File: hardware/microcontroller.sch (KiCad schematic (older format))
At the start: 8 parts, among them J1 Conn_02x05_Odd_Even, U1 ESP-WROOM-32

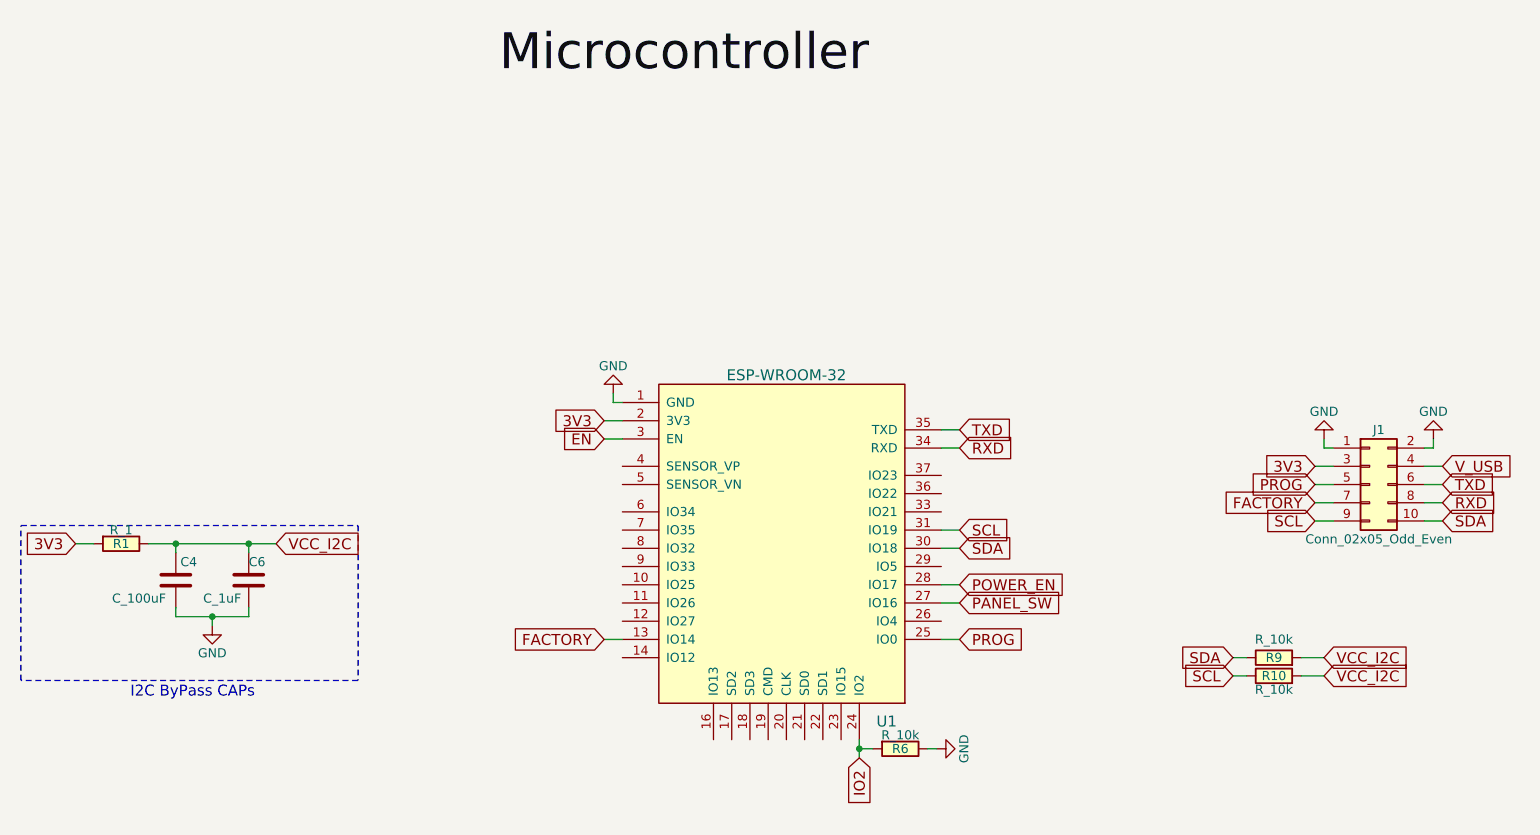
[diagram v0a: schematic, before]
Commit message: update
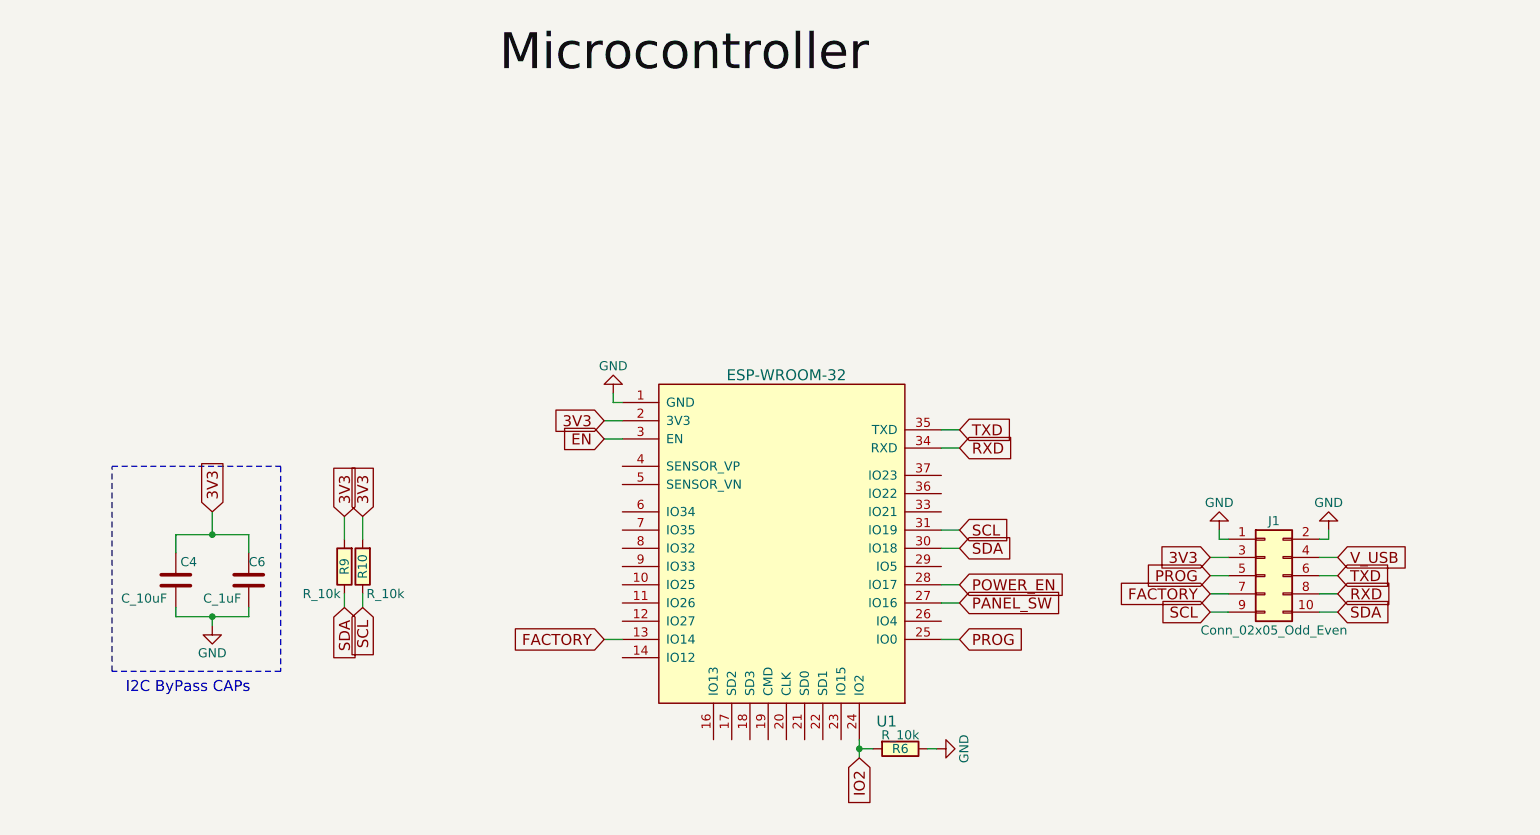
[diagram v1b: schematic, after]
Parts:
- removed C4: C_100uF, Capacitors_SMD:C_1206_HandSoldering, symbol C_100uF
- removed R1: R_1, Resistors_SMD:R_0603_HandSoldering, symbol R_1
- added C4: C_10uF, Capacitors_SMD:C_0603_HandSoldering, symbol C_10uF
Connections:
- net VCC_I2C is gone; now on net 3V3: C6.1, R10.2, R9.2
- net 3V3: now also C4.1
- net GND: now also C4.2
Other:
- moved on the sheet: J1, R10, R9
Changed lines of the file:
@@
 L GND #PWR02
 U 1 1 590979B0
-P 8725 3000
-F 0 "#PWR02" H 8725 2750 50  0001 C CNN
-F 1 "GND" H 8725 2850 50  0000 C CNN
-F 2 "" H 8725 3000 50  0000 C CNN
-F 3 "" H 8725 3000 50  0000 C CNN
-	1    8725 3000
-	-1   0    0    1
-$EndComp
-Text GLabel 8675 3150 0    60   Input ~ 0
-3V3
-Text GLabel 9375 3350 2    60   Input ~ 0
+P 8150 3500
+F 0 "#PWR02" H 8150 3250 50  0001 C CNN
+F 1 "GND" H 8150 3350 50  0000 C CNN
+F 2 "" H 8150 3500 50  0000 C CNN
+F 3 "" H 8150 3500 50  0000 C CNN
+	1    8150 3500
+	-1   0    0    1
+$EndComp
+Text GLabel 8100 3650 0    60   Input ~ 0
+3V3
+Text GLabel 8800 3850 2    60   Input ~ 0
 RXD
-Text GLabel 9375 3250 2    60   Input ~ 0
+Text GLabel 8800 3750 2    60   Input ~ 0
 TXD
-Text GLabel 9375 3150 2    60   Input ~ 0
+Text GLabel 8800 3650 2    60   Input ~ 0
 V_USB
 $Comp
 L GND #PWR03
 U 1 1 590979B2
-P 9325 3000
-F 0 "#PWR03" H 9325 2750 50  0001 C CNN
-F 1 "GND" H 9325 2850 50  0000 C CNN
-F 2 "" H 9325 3000 50  0000 C CNN
-F 3 "" H 9325 3000 50  0000 C CNN
-	1    9325 3000
-	-1   0    0    1
-$EndComp
-Wire Wire Line
-	9325 3050 9325 3000
-Wire Wire Line
-	9275 3050 9325 3050
-Wire Wire Line
-	8725 3050 8775 3050
-Wire Wire Line
-	8725 3000 8725 3050
-Wire Wire Line
-	9275 3150 9375 3150
-Wire Wire Line
-	9375 3350 9275 3350
-Wire Wire Line
-	9275 3250 9375 3250
-Wire Wire Line
-	8675 3150 8775 3150
+P 8750 3500
+F 0 "#PWR03" H 8750 3250 50  0001 C CNN
+F 1 "GND" H 8750 3350 50  0000 C CNN
+F 2 "" H 8750 3500 50  0000 C CNN
+F 3 "" H 8750 3500 50  0000 C CNN
+	1    8750 3500
+	-1   0    0    1
+$EndComp
+Wire Wire Line
+	8750 3550 8750 3500
+Wire Wire Line
+	8700 3550 8750 3550
+Wire Wire Line
+	8150 3550 8200 3550
+Wire Wire Line
+	8150 3500 8150 3550
+Wire Wire Line
+	8700 3650 8800 3650
+Wire Wire Line
+	8800 3850 8700 3850
+Wire Wire Line
+	8700 3750 8800 3750
+Wire Wire Line
+	8100 3650 8200 3650
 Wire Wire Line
 	6625 3800 6725 3800
@@
 $EndComp
 $Comp
-L C_100uF C4
-U 1 1 59C55B04
-P 2425 3775
-F 0 "C4" H 2450 3875 50  0000 L CNN
-F 1 "C_100uF" H 2075 3675 50  0000 L CNN
-F 2 "Capacitors_SMD:C_1206_HandSoldering" H 2525 4075 50  0001 C CNN
-F 3 "https://www.digikey.com/product-detail/en/tdk-corporation/C3216X5R1A107M160AC/445-6007-1-ND/2444048" H 2425 3525 50  0001 C CNN
-F 4 "C3216X5R1A107M160AC" H 2550 3975 60  0001 C CNN "Part Number"
-	1    2425 3775
-	1    0    0    -1
-$EndComp
-$Comp
 L GND #PWR04
 U 1 1 59C55B05
@@
 	1    0    0    -1
 $EndComp
-Text GLabel 1875 3575 0    60   Input ~ 0
-3V3
-Text GLabel 2975 3575 2    60   Input ~ 0
-VCC_I2C
-Wire Wire Line
-	1875 3575 1975 3575
-Wire Wire Line
-	2275 3575 2975 3575
-Wire Wire Line
-	2425 3575 2425 3625
-Wire Wire Line
-	2825 3575 2825 3625
-Connection ~ 2425 3575
-Connection ~ 2825 3575
+Text GLabel 2625 3400 1    60   Input ~ 0
+3V3
 Wire Wire Line
 	2425 3925 2425 3975
@@
 	2625 4025 2625 3975
 Connection ~ 2625 3975
-Text Notes 2175 4425 0    60   ~ 0
+Text Notes 2150 4400 0    60   ~ 0
 I2C ByPass CAPs
-Wire Notes Line
-	3425 3475 3425 4325
-Wire Notes Line
-	3425 4325 1575 4325
-Wire Notes Line
-	1575 4325 1575 3475
-Wire Notes Line
-	1575 3475 3425 3475
-Text GLabel 8675 3250 0    60   Input ~ 0
+Text GLabel 8100 3750 0    60   Input ~ 0
 PROG
-Text GLabel 8675 3350 0    60   Input ~ 0
+Text GLabel 8100 3850 0    60   Input ~ 0
 FACTORY
 Wire Wire Line
-	8675 3350 8775 3350
-Wire Wire Line
-	8675 3250 8775 3250
+	8100 3850 8200 3850
+Wire Wire Line
+	8100 3750 8200 3750
 $Comp
 L R_10k R6
@@
 Text GLabel 4775 3000 0    60   Input ~ 0
 EN
-Text GLabel 8675 3450 0    60   Input ~ 0
+Text GLabel 8100 3950 0    60   Input ~ 0
 SCL
-Text GLabel 9375 3450 2    60   Input ~ 0
+Text GLabel 8800 3950 2    60   Input ~ 0
 SDA
 Wire Wire Line
-	8675 3450 8775 3450
-Wire Wire Line
-	9275 3450 9375 3450
+	8100 3950 8200 3950
+Wire Wire Line
+	8700 3950 8800 3950
 Text GLabel 6725 3900 2    60   Input ~ 0
 PANEL_SW
@@
 L Conn_02x05_Odd_Even J1
 U 1 1 59C6C1C0
-P 8975 3250
-F 0 "J1" H 9025 3550 50  0000 C CNN
-F 1 "Conn_02x05_Odd_Even" H 9025 2950 50  0000 C CNN
-F 2 "Pin_Headers:Pin_Header_Straight_2x05_Pitch2.54mm" H 8975 3250 50  0001 C CNN
-F 3 "" H 8975 3250 50  0001 C CNN
-	1    8975 3250
-	1    0    0    -1
-$EndComp
-Text GLabel 8225 4300 0    60   Input ~ 0
+P 8400 3750
+F 0 "J1" H 8450 4050 50  0000 C CNN
+F 1 "Conn_02x05_Odd_Even" H 8450 3450 50  0000 C CNN
+F 2 "Pin_Headers:Pin_Header_Straight_2x05_Pitch2.54mm" H 8400 3750 50  0001 C CNN
+F 3 "" H 8400 3750 50  0001 C CNN
+	1    8400 3750
+	1    0    0    -1
+$EndComp
+Text GLabel 3450 3925 3    60   Input ~ 0
 SCL
-Text GLabel 8225 4200 0    60   Input ~ 0
+Text GLabel 3350 3925 3    60   Input ~ 0
 SDA
 $Comp
 L R_10k R10
 U 1 1 59C83F25
-P 8450 4300
-F 0 "R10" V 8450 4300 50  0000 C CNN
-F 1 "R_10k" V 8375 4300 50  0000 C CNN
-F 2 "Resistors_SMD:R_0603_HandSoldering" V 8380 4300 50  0001 C CNN
-F 3 "https://www.digikey.com/product-detail/en/yageo/RC0603JR-0710KL/311-10KGRCT-ND/729647" V 8530 4300 50  0001 C CNN
-F 4 "RC0603JR-0710KL" V 8630 4400 60  0001 C CNN "Part Number"
-	1    8450 4300
-	0    -1   -1   0
+P 3450 3700
+F 0 "R10" V 3450 3700 50  0000 C CNN
+F 1 "R_10k" H 3325 3850 50  0000 C CNN
+F 2 "Resistors_SMD:R_0603_HandSoldering" V 3380 3700 50  0001 C CNN
+F 3 "https://www.digikey.com/product-detail/en/yageo/RC0603JR-0710KL/311-10KGRCT-ND/729647" V 3530 3700 50  0001 C CNN
+F 4 "RC0603JR-0710KL" V 3630 3800 60  0001 C CNN "Part Number"
+	1    3450 3700
+	-1   0    0    1
 $EndComp
 $Comp
 L R_10k R9
 U 1 1 59C83F7C
-P 8450 4200
-F 0 "R9" V 8450 4200 50  0000 C CNN
-F 1 "R_10k" V 8550 4200 50  0000 C CNN
-F 2 "Resistors_SMD:R_0603_HandSoldering" V 8380 4200 50  0001 C CNN
-F 3 "https://www.digikey.com/product-detail/en/yageo/RC0603JR-0710KL/311-10KGRCT-ND/729647" V 8530 4200 50  0001 C CNN
-F 4 "RC0603JR-0710KL" V 8630 4300 60  0001 C CNN "Part Number"
-	1    8450 4200
-	0    -1   -1   0
-$EndComp
-Wire Wire Line
-	8300 4300 8225 4300
-Wire Wire Line
-	8225 4200 8300 4200
-Wire Wire Line
-	8600 4200 8725 4200
-Wire Wire Line
-	8725 4300 8600 4300
-Text GLabel 8725 4200 2    60   Input ~ 0
-VCC_I2C
-Text GLabel 8725 4300 2    60   Input ~ 0
-VCC_I2C
-$Comp
-L R_1 R1
-U 1 1 59E3C91A
-P 2125 3575
-F 0 "R1" V 2125 3575 50  0000 C CNN
-F 1 "R_1" V 2050 3575 50  0000 C CNN
-F 2 "Resistors_SMD:R_0603_HandSoldering" V 2055 3575 50  0001 C CNN
-F 3 "https://www.digikey.com/product-detail/en/stackpole-electronics-inc/RNCP0603FTD1R00/RNCP0603FTD1R00CT-ND/2240411" V 2205 3575 50  0001 C CNN
-F 4 "RNCP0603FTD1R00" V 2305 3675 60  0001 C CNN "Part Number"
-	1    2125 3575
-	0    1    1    0
-$EndComp
+P 3350 3700
+F 0 "R9" V 3350 3700 50  0000 C CNN
+F 1 "R_10k" H 3475 3850 50  0000 C CNN
+F 2 "Resistors_SMD:R_0603_HandSoldering" V 3280 3700 50  0001 C CNN
+F 3 "https://www.digikey.com/product-detail/en/yageo/RC0603JR-0710KL/311-10KGRCT-ND/729647" V 3430 3700 50  0001 C CNN
+F 4 "RC0603JR-0710KL" V 3530 3800 60  0001 C CNN "Part Number"
+	1    3350 3700
+	-1   0    0    1
+$EndComp
+Wire Wire Line
+	3450 3850 3450 3925
+Wire Wire Line
+	3350 3925 3350 3850
+Wire Wire Line
+	3350 3550 3350 3425
+Wire Wire Line
+	3450 3425 3450 3550
+Text GLabel 3350 3425 1    60   Input ~ 0
+3V3
+Text GLabel 3450 3425 1    60   Input ~ 0
+3V3
+$Comp
+L C_10uF C4
+U 1 1 5A10664F
+P 2425 3775
+F 0 "C4" H 2450 3875 50  0000 L CNN
+F 1 "C_10uF" H 2125 3675 50  0000 L CNN
+F 2 "Capacitors_SMD:C_0603_HandSoldering" H 2525 4075 50  0001 C CNN
+F 3 "https://www.digikey.com/product-detail/en/murata-electronics-north-america/GRM188R61A106ME69D/490-10475-1-ND/5026393" H 2425 3525 50  0001 C CNN
+F 4 "GRM188R61A106ME69D" H 2550 3975 60  0001 C CNN "Part Number"
+	1    2425 3775
+	1    0    0    -1
+$EndComp
+Wire Wire Line
+	2425 3625 2425 3525
+Wire Wire Line
+	2425 3525 2825 3525
+Wire Wire Line
+	2625 3525 2625 3400
+Wire Wire Line
+	2825 3525 2825 3625
+Connection ~ 2625 3525
+Wire Notes Line
+	2075 4275 2075 3150
+Wire Notes Line
+	2075 3150 3000 3150
+Wire Notes Line
+	3000 3150 3000 4275
+Wire Notes Line
+	3000 4275 2075 4275
 $EndSCHEMATC
